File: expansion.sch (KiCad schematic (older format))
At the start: 3 parts, among them J7 DF40HC(3.5)-60DS, J9 DF40HC(3.5)-60DS, U1 IMX8MM

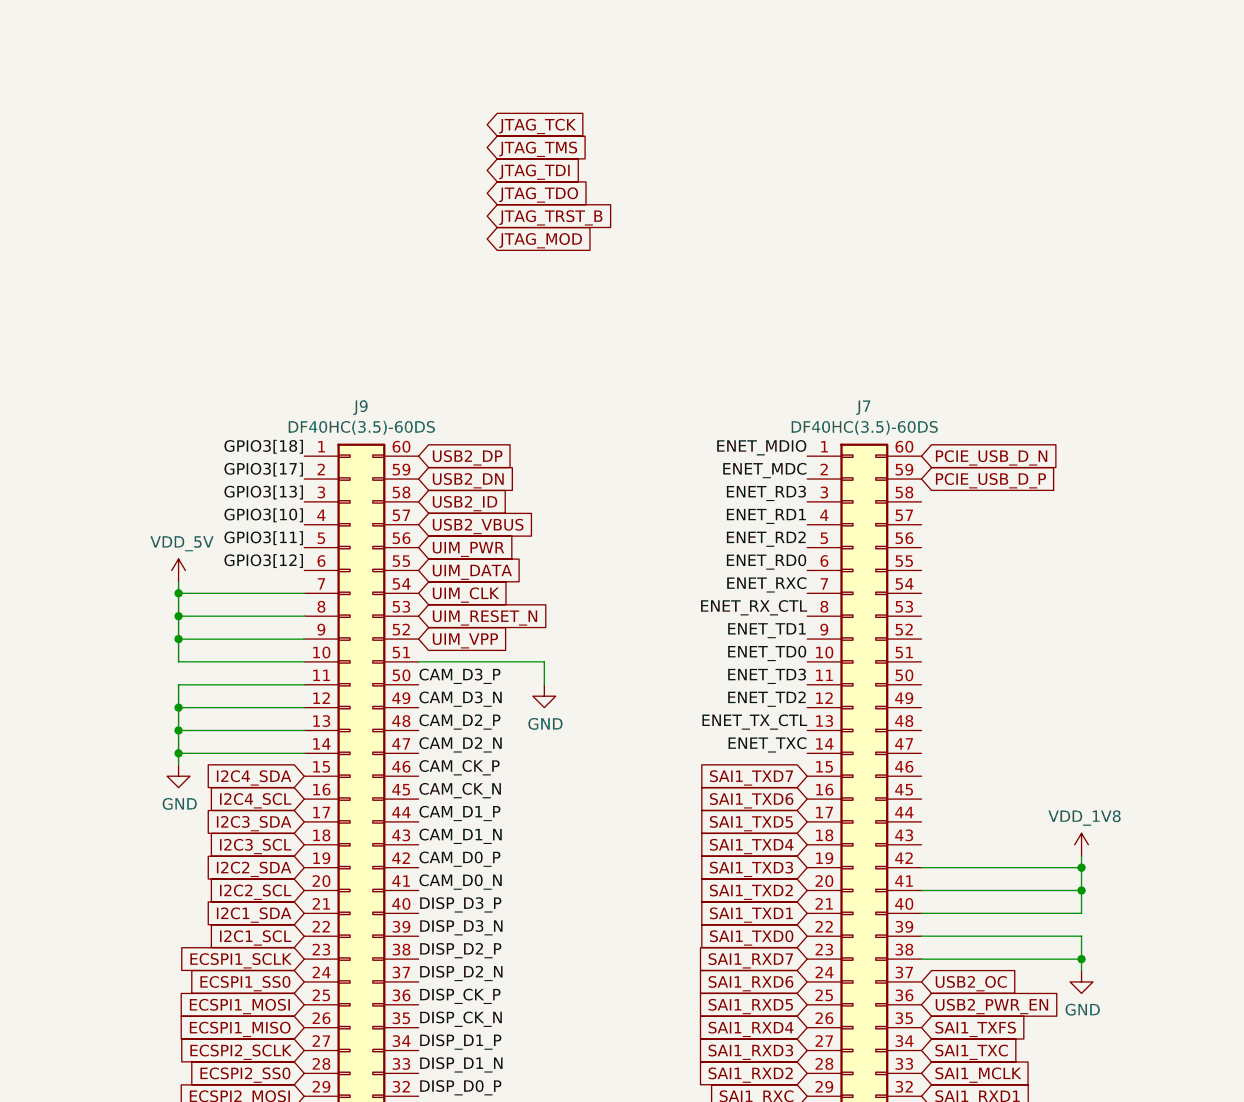
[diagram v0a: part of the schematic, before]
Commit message: Finish remaining routing
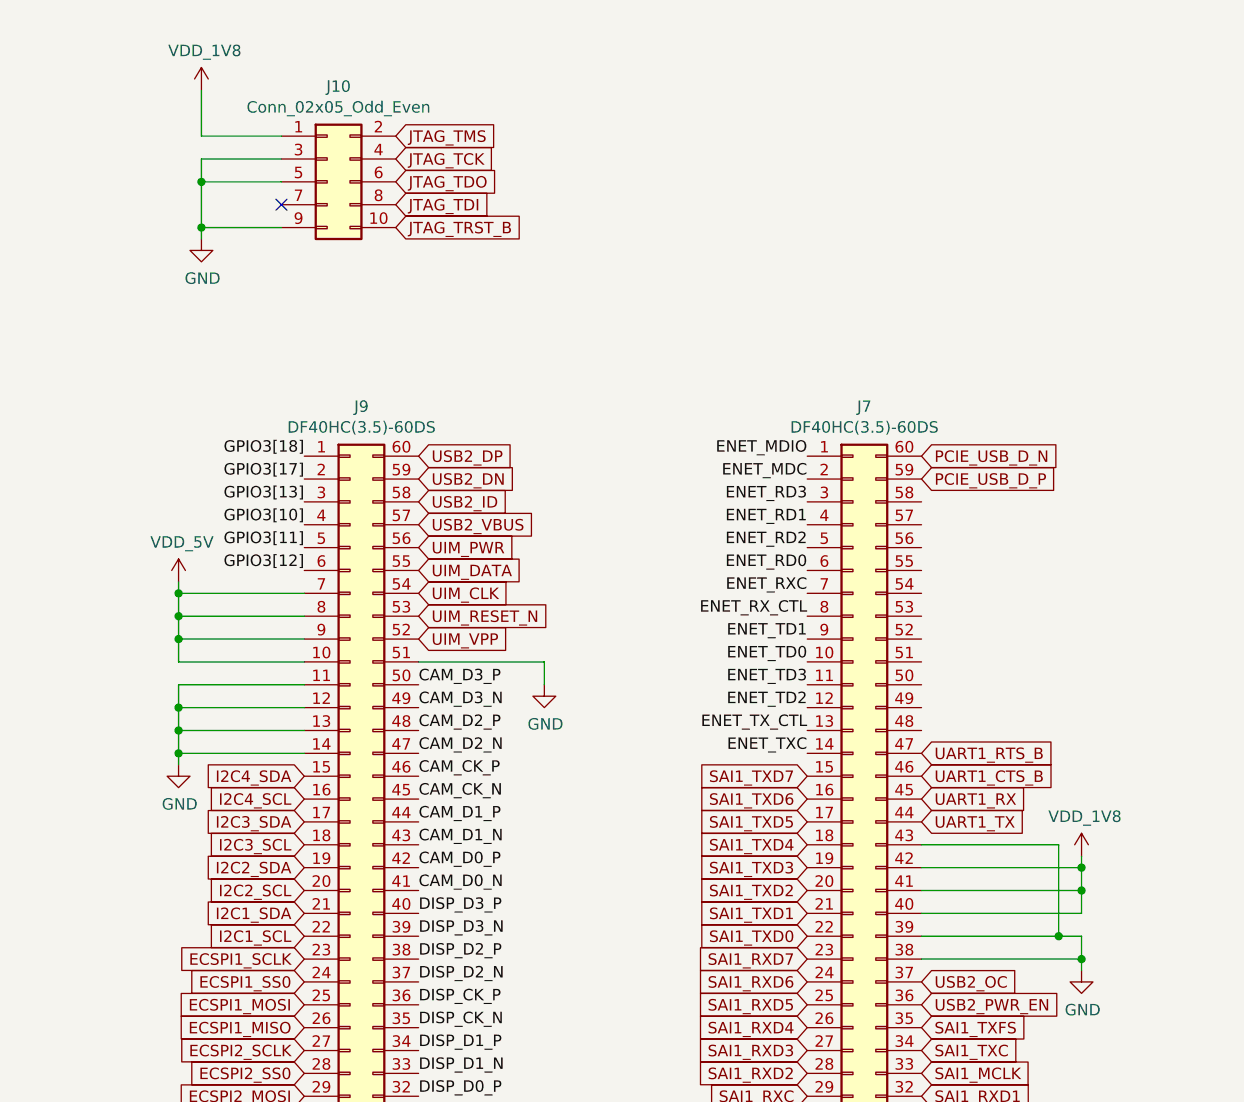
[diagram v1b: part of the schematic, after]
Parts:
- added J10: Conn_02x05_Odd_Even, Connector_PinHeader_1.27mm:PinHeader_2x05_P1.27mm_Vertical_SMD, symbol Connector_Generic:Conn_02x05_Odd_Even
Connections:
- net GND: now also J7.43 (Pin_43), J10.3 (Pin_3), J10.5 (Pin_5), J10.9 (Pin_9)
- net JTAG_TCK: now also J10.4 (Pin_4)
- net JTAG_TDI: now also J10.8 (Pin_8)
- net JTAG_TDO: now also J10.6 (Pin_6)
- net JTAG_TMS: now also J10.2 (Pin_2)
- net JTAG_TRST_B: now also J10.10 (Pin_10)
- net VDD_1V8: now also J10.1 (Pin_1)
- net UART1_TX: now reaches J7.44 (Pin_44)
- net UART1_RX: now reaches J7.45 (Pin_45)
- net UART1_CTS_B: now reaches J7.46 (Pin_46)
- net UART1_RTS_B: now reaches J7.47 (Pin_47)
- no-connect marks 0 -> 1
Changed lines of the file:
@@
 	1    0    0    -1
 $EndComp
-Text GLabel 5350 1100 2    50   Input ~ 0
+Text GLabel 4950 1250 2    50   Input ~ 0
 JTAG_TCK
-Text GLabel 5350 1200 2    50   Input ~ 0
+Text GLabel 4950 1150 2    50   Input ~ 0
 JTAG_TMS
-Text GLabel 5350 1300 2    50   Input ~ 0
+Text GLabel 4950 1450 2    50   Input ~ 0
 JTAG_TDI
-Text GLabel 5350 1400 2    50   Input ~ 0
+Text GLabel 4950 1350 2    50   Input ~ 0
 JTAG_TDO
-Text GLabel 5350 1500 2    50   Input ~ 0
+Text GLabel 4950 1550 2    50   Input ~ 0
 JTAG_TRST_B
-Text GLabel 5350 1600 2    50   Input ~ 0
-JTAG_MOD
 $Comp
 L mxenc:MIMX8MM6DVTLZAA U1
@@
 	7950 4750 7250 4750
 Wire Wire Line
-	7250 4650 7950 4650
+	7250 4650 7850 4650
 Wire Wire Line
 	7950 4650 7950 4750
@@
 Text GLabel 7250 2650 2    50   Input ~ 0
 PCIE_USB_D_P
+Text GLabel 7250 3950 2    50   Input ~ 0
+UART1_CTS_B
+Text GLabel 7250 3850 2    50   Input ~ 0
+UART1_RTS_B
+Text GLabel 7250 4050 2    50   Input ~ 0
+UART1_RX
+Text GLabel 7250 4150 2    50   Input ~ 0
+UART1_TX
+Wire Wire Line
+	7250 4250 7850 4250
+Wire Wire Line
+	7850 4250 7850 4650
+Connection ~ 7850 4650
+Wire Wire Line
+	7850 4650 7950 4650
+$Comp
+L Connector_Generic:Conn_02x05_Odd_Even J10
+U 1 1 5EC3A2D4
+P 4650 1350
+F 0 "J10" H 4700 1767 50  0000 C CNN
+F 1 "Conn_02x05_Odd_Even" H 4700 1676 50  0000 C CNN
+F 2 "Connector_PinHeader_1.27mm:PinHeader_2x05_P1.27mm_Vertical_SMD" H 4650 1350 50  0001 C CNN
+F 3 "~" H 4650 1350 50  0001 C CNN
+	1    4650 1350
+	1    0    0    -1
+$EndComp
+$Comp
+L power:GND #PWR0239
+U 1 1 5EC40863
+P 4100 1600
+F 0 "#PWR0239" H 4100 1350 50  0001 C CNN
+F 1 "GND" H 4105 1427 50  0000 C CNN
+F 2 "" H 4100 1600 50  0001 C CNN
+F 3 "" H 4100 1600 50  0001 C CNN
+	1    4100 1600
+	1    0    0    -1
+$EndComp
+Wire Wire Line
+	4100 1600 4100 1550
+Wire Wire Line
+	4100 1350 4450 1350
+Wire Wire Line
+	4450 1250 4100 1250
+Wire Wire Line
+	4100 1250 4100 1350
+Connection ~ 4100 1350
+Wire Wire Line
+	4450 1550 4100 1550
+Connection ~ 4100 1550
+Wire Wire Line
+	4100 1550 4100 1350
+NoConn ~ 4450 1450
+$Comp
+L mxenc:VDD_1V8 #PWR0244
+U 1 1 5ED1315B
+P 4100 950
+F 0 "#PWR0244" H 4100 800 50  0001 C CNN
+F 1 "VDD_1V8" H 4115 1123 50  0000 C CNN
+F 2 "" H 4100 950 50  0001 C CNN
+F 3 "" H 4100 950 50  0001 C CNN
+	1    4100 950
+	1    0    0    -1
+$EndComp
+Wire Wire Line
+	4100 950  4100 1150
+Wire Wire Line
+	4100 1150 4450 1150
 $EndSCHEMATC

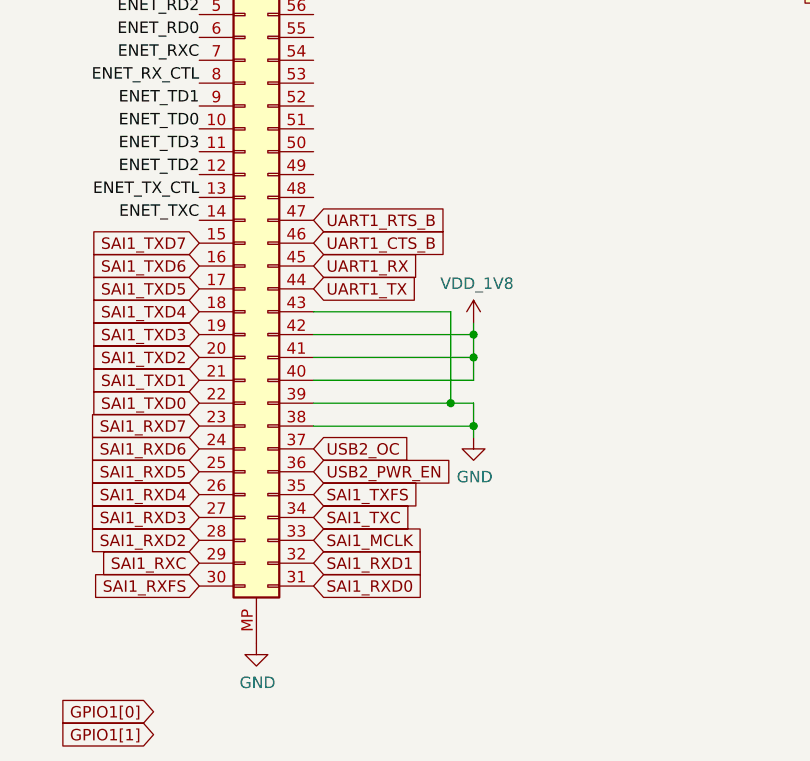
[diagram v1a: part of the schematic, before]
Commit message: wip more uart routing
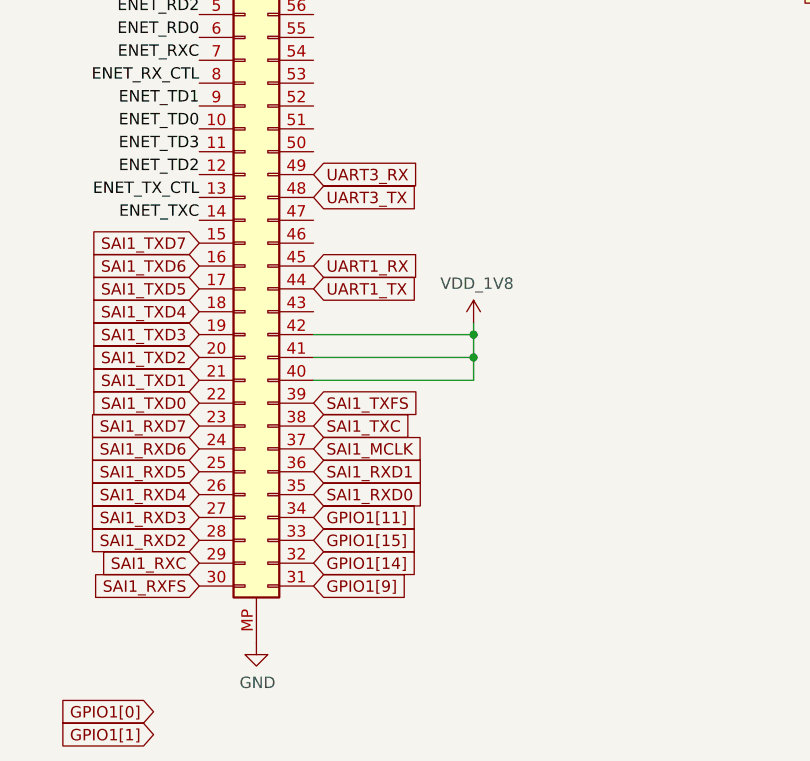
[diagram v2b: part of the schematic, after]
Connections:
- net USB2_OC is gone; now on net SAI1_MCLK: J7.37 (Pin_37)
- net USB2_PWR_EN is gone; now on net SAI1_RXD1: J7.36 (Pin_36)
- net GND: no longer J7.38 (Pin_38), J7.39 (Pin_39), J7.43 (Pin_43)
- net SAI1_MCLK: no longer J7.33 (Pin_33)
- net SAI1_RXD0: now also J7.35 (Pin_35); no longer J7.31 (Pin_31)
- net SAI1_RXD1: no longer J7.32 (Pin_32)
- net SAI1_TXC: now also J7.38 (Pin_38); no longer J7.34 (Pin_34)
- net SAI1_TXFS: now also J7.39 (Pin_39); no longer J7.35 (Pin_35)
- net UART3_TX: now reaches J7.48 (Pin_48)
- net UART3_RX: now reaches J7.49 (Pin_49)
- net UART1_CTS_B: no longer names the net of J7.46 (Pin_46)
- net UART1_RTS_B: no longer names the net of J7.47 (Pin_47)
- new net GPIO1[11]: J7.34 (Pin_34)
- new net GPIO1[14]: J7.32 (Pin_32)
- new net GPIO1[15]: J7.33 (Pin_33)
- new net GPIO1[9]: J7.31 (Pin_31)
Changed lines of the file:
@@
 Text GLabel 6750 5450 0    50   Input ~ 0
 SAI1_RXFS
-Text GLabel 7250 5350 2    50   Input ~ 0
+Text GLabel 7250 4950 2    50   Input ~ 0
 SAI1_RXD1
-Text GLabel 7250 5450 2    50   Input ~ 0
+Text GLabel 7250 5050 2    50   Input ~ 0
 SAI1_RXD0
-Text GLabel 7250 5150 2    50   Input ~ 0
+Text GLabel 7250 4750 2    50   Input ~ 0
 SAI1_TXC
-Text GLabel 7250 5050 2    50   Input ~ 0
+Text GLabel 7250 4650 2    50   Input ~ 0
 SAI1_TXFS
-Text GLabel 7250 5250 2    50   Input ~ 0
+Text GLabel 7250 4850 2    50   Input ~ 0
 SAI1_MCLK
 Text Label 2750 2800 0    50   ~ 0
@@
 Text GLabel 2750 1900 2    50   Input ~ 0
 BTN1
-Text GLabel 7250 4850 2    50   Input ~ 0
-USB2_OC
-Text GLabel 7250 4950 2    50   Input ~ 0
-USB2_PWR_EN
 Text GLabel 4550 5150 0    50   Input ~ 0
 ECSPI2_SCLK
@@
 Connection ~ 4000 3650
 $Comp
-L power:GND #PWR0222
-U 1 1 5F468948
-P 7950 4800
-F 0 "#PWR0222" H 7950 4550 50  0001 C CNN
-F 1 "GND" H 7955 4627 50  0000 C CNN
-F 2 "" H 7950 4800 50  0001 C CNN
-F 3 "" H 7950 4800 50  0001 C CNN
-	1    7950 4800
-	1    0    0    -1
-$EndComp
-Wire Wire Line
-	7950 4800 7950 4750
-Wire Wire Line
-	7950 4750 7250 4750
-Wire Wire Line
-	7250 4650 7850 4650
-Wire Wire Line
-	7950 4650 7950 4750
-Connection ~ 7950 4750
-$Comp
 L mxenc:VDD_1V8 #PWR0223
 U 1 1 5F46F757
@@
 Text GLabel 7250 2650 2    50   Input ~ 0
 PCIE_USB_D_P
-Text GLabel 7250 3950 2    50   Input ~ 0
-UART1_CTS_B
-Text GLabel 7250 3850 2    50   Input ~ 0
-UART1_RTS_B
+Text GLabel 7250 3750 2    50   Input ~ 0
+UART3_TX
+Text GLabel 7250 3650 2    50   Input ~ 0
+UART3_RX
 Text GLabel 7250 4050 2    50   Input ~ 0
 UART1_RX
 Text GLabel 7250 4150 2    50   Input ~ 0
 UART1_TX
-Wire Wire Line
-	7250 4250 7850 4250
-Wire Wire Line
-	7850 4250 7850 4650
-Connection ~ 7850 4650
-Wire Wire Line
-	7850 4650 7950 4650
 $Comp
 L Connector_Generic:Conn_02x05_Odd_Even J10
@@
 Wire Wire Line
 	4100 1150 4450 1150
+Text GLabel 7250 5450 2    50   Input ~ 0
+GPIO1[9]
+Text GLabel 7250 5150 2    50   Input ~ 0
+GPIO1[11]
+Text GLabel 7250 5350 2    50   Input ~ 0
+GPIO1[14]
+Text GLabel 7250 5250 2    50   Input ~ 0
+GPIO1[15]
 $EndSCHEMATC
